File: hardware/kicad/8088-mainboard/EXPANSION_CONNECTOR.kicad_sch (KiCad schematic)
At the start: 3 parts, among them J1 Exp0, J3 Exp1, J4 Exp2

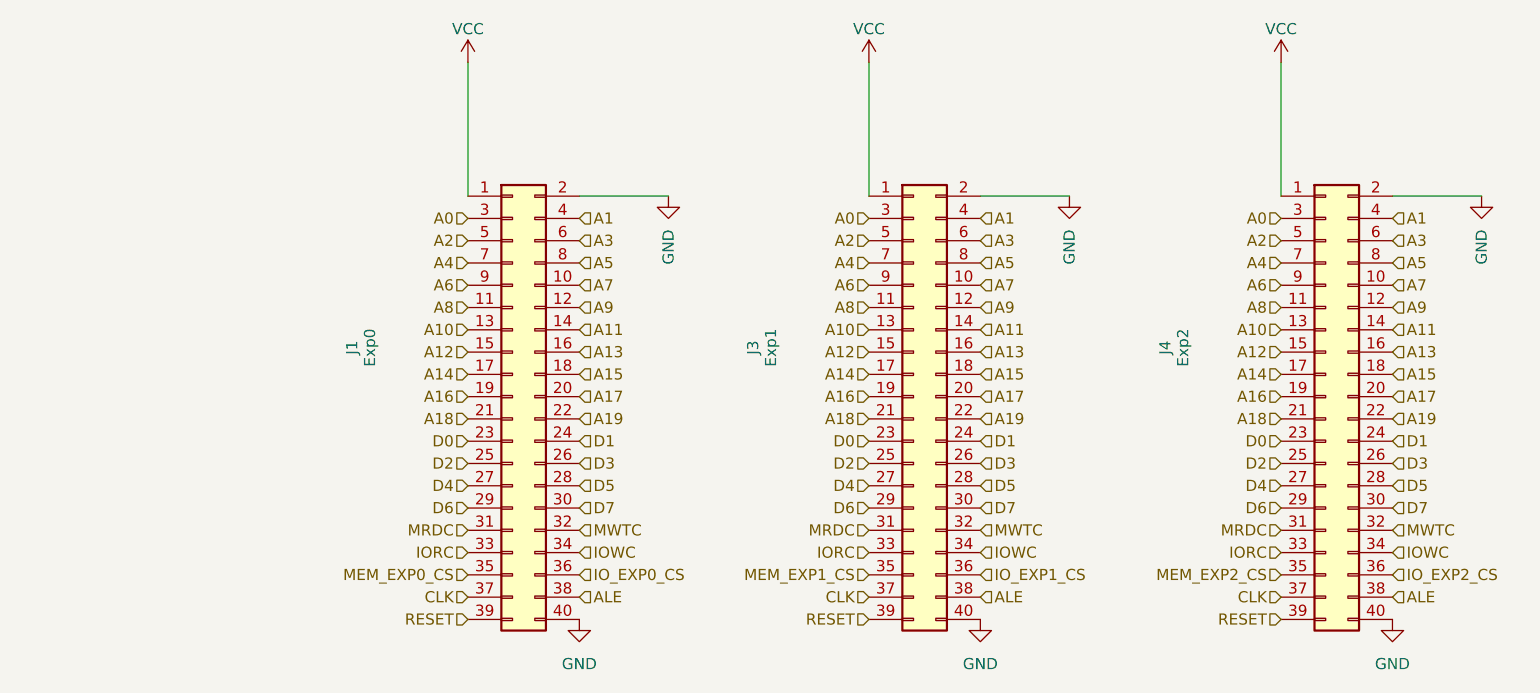
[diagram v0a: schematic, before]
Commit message: Add PSB board design
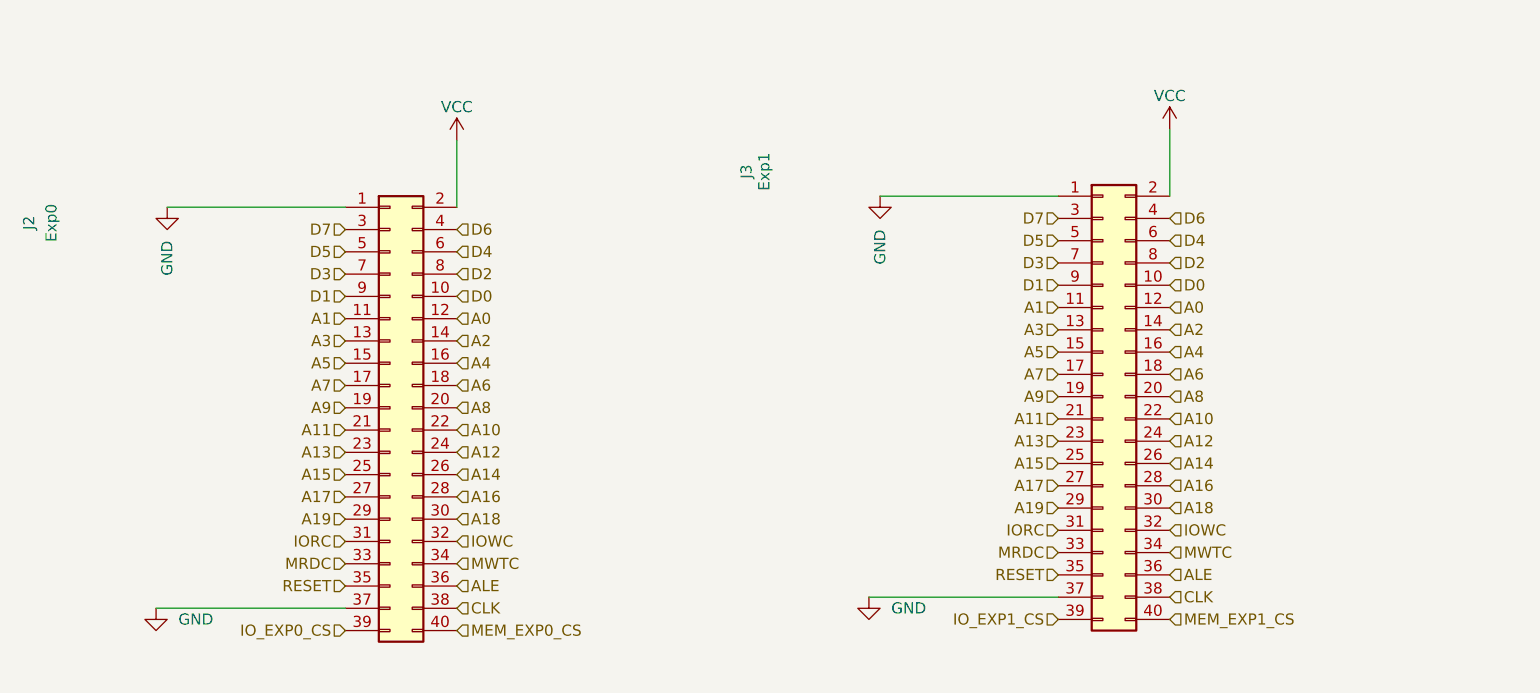
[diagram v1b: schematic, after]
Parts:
- removed J4: Exp2, Connector_IDC:IDC-Header_2x20_P2.54mm_Vertical, symbol Connector_Generic:Conn_02x20_Odd_Even
- renumbered J1 to J2
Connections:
- net A0: now also J2.12 (Pin_12), J3.12 (Pin_12); no longer J2.3 (Pin_3), J3.3 (Pin_3)
- net A1: now also J2.11 (Pin_11), J3.11 (Pin_11); no longer J2.4 (Pin_4), J3.4 (Pin_4)
- net A10: now also J2.22 (Pin_22), J3.22 (Pin_22); no longer J2.13 (Pin_13), J3.13 (Pin_13)
- net A11: now also J2.21 (Pin_21), J3.21 (Pin_21); no longer J2.14 (Pin_14), J3.14 (Pin_14)
- net A12: now also J2.24 (Pin_24), J3.24 (Pin_24); no longer J2.15 (Pin_15), J3.15 (Pin_15)
- net A13: now also J2.23 (Pin_23), J3.23 (Pin_23); no longer J2.16 (Pin_16), J3.16 (Pin_16)
- net A14: now also J2.26 (Pin_26), J3.26 (Pin_26); no longer J2.17 (Pin_17), J3.17 (Pin_17)
- net A15: now also J2.25 (Pin_25), J3.25 (Pin_25); no longer J2.18 (Pin_18), J3.18 (Pin_18)
- net A16: now also J2.28 (Pin_28), J3.28 (Pin_28); no longer J2.19 (Pin_19), J3.19 (Pin_19)
- net A17: now also J2.27 (Pin_27), J3.27 (Pin_27); no longer J2.20 (Pin_20), J3.20 (Pin_20)
- net A18: now also J2.30 (Pin_30), J3.30 (Pin_30); no longer J2.21 (Pin_21), J3.21 (Pin_21)
- net A19: now also J2.29 (Pin_29), J3.29 (Pin_29); no longer J2.22 (Pin_22), J3.22 (Pin_22)
- net A2: now also J2.14 (Pin_14), J3.14 (Pin_14); no longer J2.5 (Pin_5), J3.5 (Pin_5)
- net A3: now also J2.13 (Pin_13), J3.13 (Pin_13); no longer J2.6 (Pin_6), J3.6 (Pin_6)
- net A4: now also J2.16 (Pin_16), J3.16 (Pin_16); no longer J2.7 (Pin_7), J3.7 (Pin_7)
- net A5: now also J2.15 (Pin_15), J3.15 (Pin_15); no longer J2.8 (Pin_8), J3.8 (Pin_8)
- net A6: now also J2.18 (Pin_18), J3.18 (Pin_18); no longer J2.9 (Pin_9), J3.9 (Pin_9)
- net A7: now also J2.17 (Pin_17), J3.17 (Pin_17); no longer J2.10 (Pin_10), J3.10 (Pin_10)
- net A8: now also J2.20 (Pin_20), J3.20 (Pin_20); no longer J2.11 (Pin_11), J3.11 (Pin_11)
- net A9: now also J2.19 (Pin_19), J3.19 (Pin_19); no longer J2.12 (Pin_12), J3.12 (Pin_12)
- net ALE: now also J2.36 (Pin_36), J3.36 (Pin_36); no longer J2.38 (Pin_38), J3.38 (Pin_38)
- net CLK: now also J2.38 (Pin_38), J3.38 (Pin_38); no longer J2.37 (Pin_37), J3.37 (Pin_37)
- net D0: now also J2.10 (Pin_10), J3.10 (Pin_10); no longer J2.23 (Pin_23), J3.23 (Pin_23)
- net D1: now also J2.9 (Pin_9), J3.9 (Pin_9); no longer J2.24 (Pin_24), J3.24 (Pin_24)
- net D2: now also J2.8 (Pin_8), J3.8 (Pin_8); no longer J2.25 (Pin_25), J3.25 (Pin_25)
- net D3: now also J2.7 (Pin_7), J3.7 (Pin_7); no longer J2.26 (Pin_26), J3.26 (Pin_26)
- net D4: now also J2.6 (Pin_6), J3.6 (Pin_6); no longer J2.27 (Pin_27), J3.27 (Pin_27)
- net D5: now also J2.5 (Pin_5), J3.5 (Pin_5); no longer J2.28 (Pin_28), J3.28 (Pin_28)
- net D6: now also J2.4 (Pin_4), J3.4 (Pin_4); no longer J2.29 (Pin_29), J3.29 (Pin_29)
- net D7: now also J2.3 (Pin_3), J3.3 (Pin_3); no longer J2.30 (Pin_30), J3.30 (Pin_30)
- net GND: now also J2.1 (Pin_1), J2.37 (Pin_37), J3.1 (Pin_1), J3.37 (Pin_37); no longer J2.2 (Pin_2), J2.40 (Pin_40), J3.2 (Pin_2), J3.40 (Pin_40)
- net IORC: now also J2.31 (Pin_31), J3.31 (Pin_31); no longer J2.33 (Pin_33), J3.33 (Pin_33)
- net IOWC: now also J2.32 (Pin_32), J3.32 (Pin_32); no longer J2.34 (Pin_34), J3.34 (Pin_34)
- net IO_EXP0_CS: now also J2.39 (Pin_39); no longer J2.36 (Pin_36)
- net IO_EXP1_CS: now also J3.39 (Pin_39); no longer J3.36 (Pin_36)
- net MEM_EXP0_CS: now also J2.40 (Pin_40); no longer J2.35 (Pin_35)
- net MEM_EXP1_CS: now also J3.40 (Pin_40); no longer J3.35 (Pin_35)
- net MRDC: now also J2.33 (Pin_33), J3.33 (Pin_33); no longer J2.31 (Pin_31), J3.31 (Pin_31)
- net MWTC: now also J2.34 (Pin_34), J3.34 (Pin_34); no longer J2.32 (Pin_32), J3.32 (Pin_32)
- net RESET: now also J2.35 (Pin_35), J3.35 (Pin_35); no longer J2.39 (Pin_39), J3.39 (Pin_39)
- net VCC: now also J2.2 (Pin_2), J3.2 (Pin_2); no longer J2.1 (Pin_1), J3.1 (Pin_1)
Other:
- moved on the sheet: J2, J3
